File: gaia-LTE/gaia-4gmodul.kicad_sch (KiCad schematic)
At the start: 24 parts, among them J1 4G antenna connector(U.FL), J6 Global Connector Technology S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, Q1 DTC143ZEBTL, Q3 DTC143ZEBTL, Q4 DTC143ZEBTL, U1 SIM7600E-H, U2 Gaia Connector A, U3 Gaia Connector B

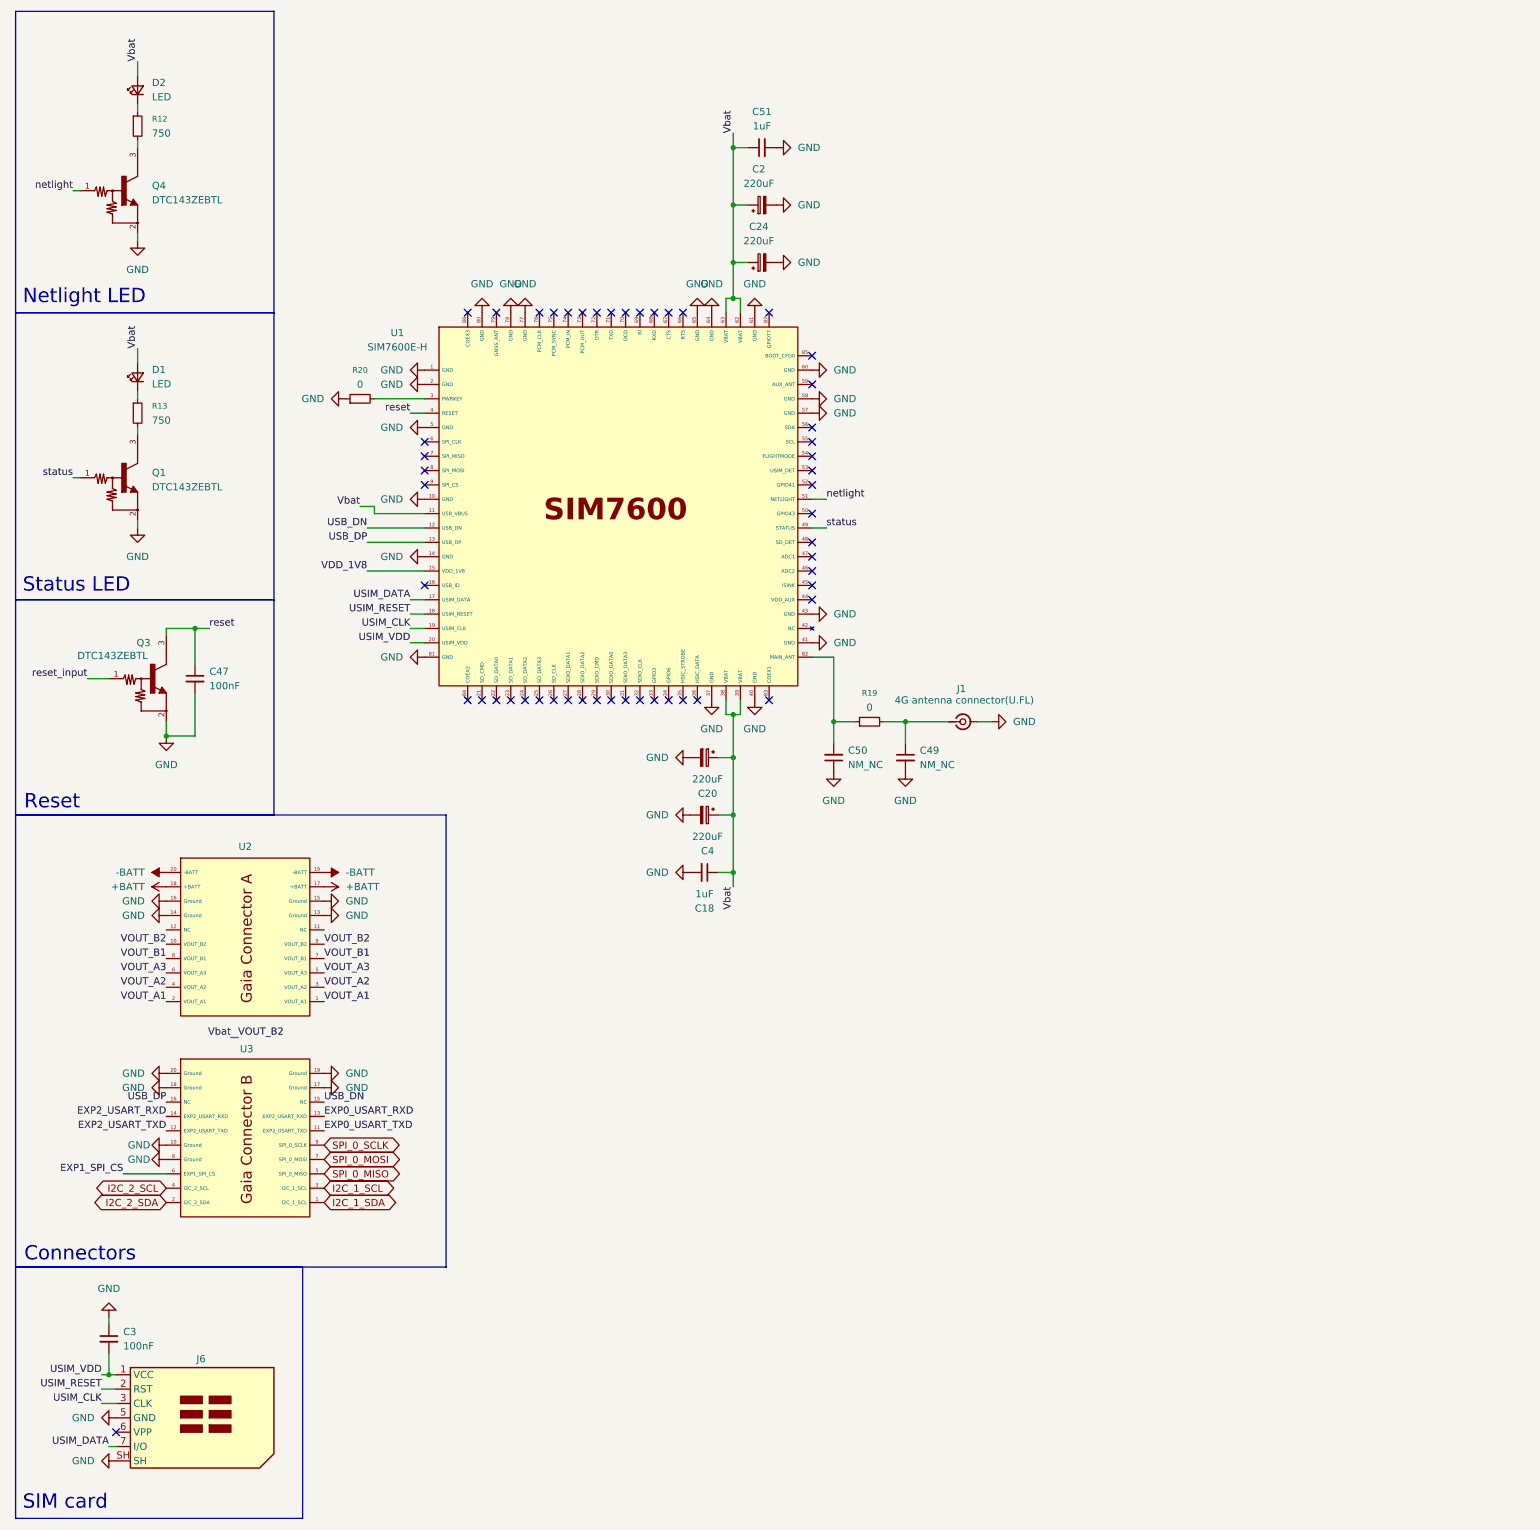
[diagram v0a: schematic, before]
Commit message: -
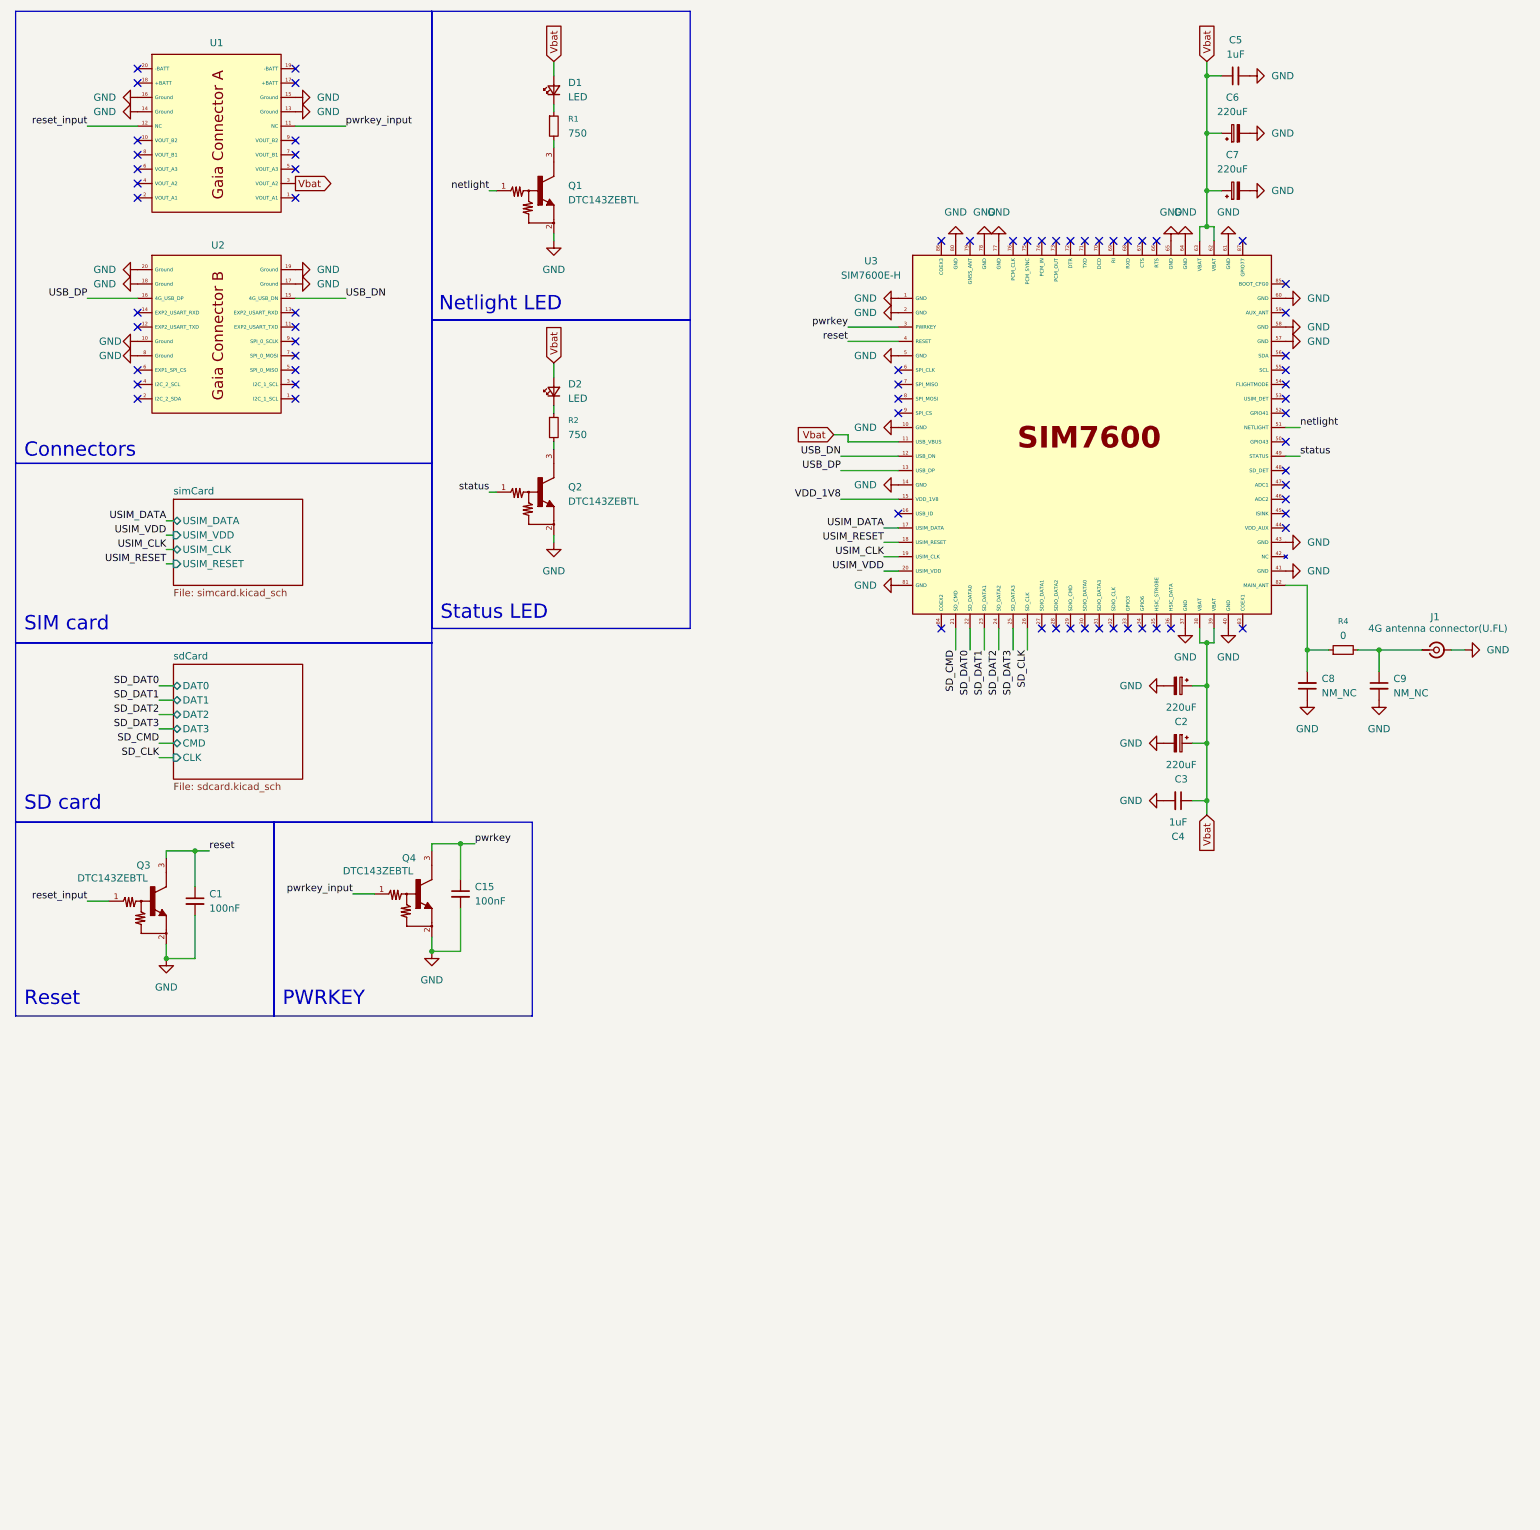
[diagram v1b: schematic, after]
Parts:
- removed C3: 100nF, Capacitor_SMD:C_0402_1005Metric, symbol Device:C_Small
- removed J6: Global Connector Technology SIM8060-6-0-14-00-A, Connector_Card:nanoSIM_GCT_SIM8060-6-0-14-00, symbol Connector:SIM_Card_Shielded
- removed R20: 0, Resistor_SMD:R_0603_1608Metric, symbol Device:R_Small
- added C15: 100nF, Capacitor_SMD:C_0603_1608Metric, symbol Device:C_Small
- added Q4: DTC143ZEBTL, gaia-4gmodul-footprints:DTC143ZEBTL, symbol gaia-4gmodul-symbols:DTC143ZEBTL
- U1: renamed from U2; footprint gaia-4gmodul-footprints:Gaia_connector_4_6layer -> gaia-4gmodul-footprints:Gaia_connector_2_4layer
- U2: renamed from U3; footprint gaia-4gmodul-footprints:Gaia_connector_4_6layer -> gaia-4gmodul-footprints:Gaia_connector_2_4layer
- renumbered C47 to C1, C20 to C2, C4 to C3, C18 to C4, C51 to C5, C2 to C6, C24 to C7, C50 to C8, C49 to C9, D2 to D1, D1 to D2, Q4 to Q1, Q1 to Q2, R12 to R1, R13 to R2, R19 to R4, U1 to U3
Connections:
- net GND: now also C15.2, Q4.2
- net reset_input: now also U1.12 (NC)
- net SD_CMD: now reaches U3.21 (SD_CMD)
- net SD_DAT0: now reaches U3.22 (SD_DATA0)
- net SD_DAT1: now reaches U3.23 (SD_DATA1)
- net SD_DAT2: now reaches U3.24 (SD_DATA2)
- net SD_DAT3: now reaches U3.25 (SD_DATA3)
- net SD_CLK: now reaches U3.26 (SD_CLK)
- net pwrkey: now reaches U3.3 (PWRKEY)
- net pwrkey: now also C15.1, Q4.3
- net pwrkey_input: now reaches U1.11 (NC)
- net pwrkey_input: now also Q4.1
- net +BATT: no longer names the net of U1.17 (+BATT)
- net +BATT: no longer U1.18 (+BATT)
- net -BATT: no longer names the net of U1.19 (-BATT)
- net -BATT: no longer U1.20 (-BATT)
- net EXP0_USART_RXD: no longer names the net of U2.13 (EXP2_USART_RXD)
- net EXP0_USART_TXD: no longer names the net of U2.11 (EXP2_USART_TXD)
- net EXP1_SPI_CS: no longer names the net of U2.6 (EXP1_SPI_CS)
- net EXP2_USART_RXD: no longer names the net of U2.14 (EXP2_USART_RXD)
- net EXP2_USART_TXD: no longer names the net of U2.12 (EXP2_USART_TXD)
- net I2C_1_SCL: no longer names the net of U2.3 (I2C_1_SCL)
- net I2C_1_SDA: no longer names the net of U2.1 (I2C_1_SCL)
- net I2C_2_SCL: no longer names the net of U2.4 (I2C_2_SCL)
- net I2C_2_SDA: no longer names the net of U2.2 (I2C_2_SDA)
- net SPI_0_MISO: no longer names the net of U2.5 (SPI_0_MISO)
- net SPI_0_MOSI: no longer names the net of U2.7 (SPI_0_MOSI)
- net SPI_0_SCLK: no longer names the net of U2.9 (SPI_0_SCLK)
- net VOUT_A1: no longer names the net of U1.1 (VOUT_A1)
- net VOUT_A1: no longer U1.2 (VOUT_A1)
- net VOUT_A2: no longer names the net of U1.4 (VOUT_A2)
- net VOUT_A2: no longer U1.3 (VOUT_A2)
- net VOUT_A3: no longer names the net of U1.5 (VOUT_A3)
- net VOUT_A3: no longer U1.6 (VOUT_A3)
- net VOUT_B1: no longer names the net of U1.7 (VOUT_B1)
- net VOUT_B1: no longer U1.8 (VOUT_B1)
- net VOUT_B2 renamed Vbat
- net Vbat: now also U1.3 (VOUT_A2); no longer U1.10 (VOUT_B2), U1.9 (VOUT_B2)
- no-connect marks 51 -> 69
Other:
- added sheet sdCard (sdcard.kicad_sch)
- added sheet simCard (simcard.kicad_sch)
- note added: "PWRKEY"
- note added: "SD card"
- moved on the sheet: C1, C2, C3, C4, C5, C6, C7, C8, C9, D1, D2, J1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
